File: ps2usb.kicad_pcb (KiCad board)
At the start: 2 copper layers, 62.6 x 48.2 mm, 13 parts

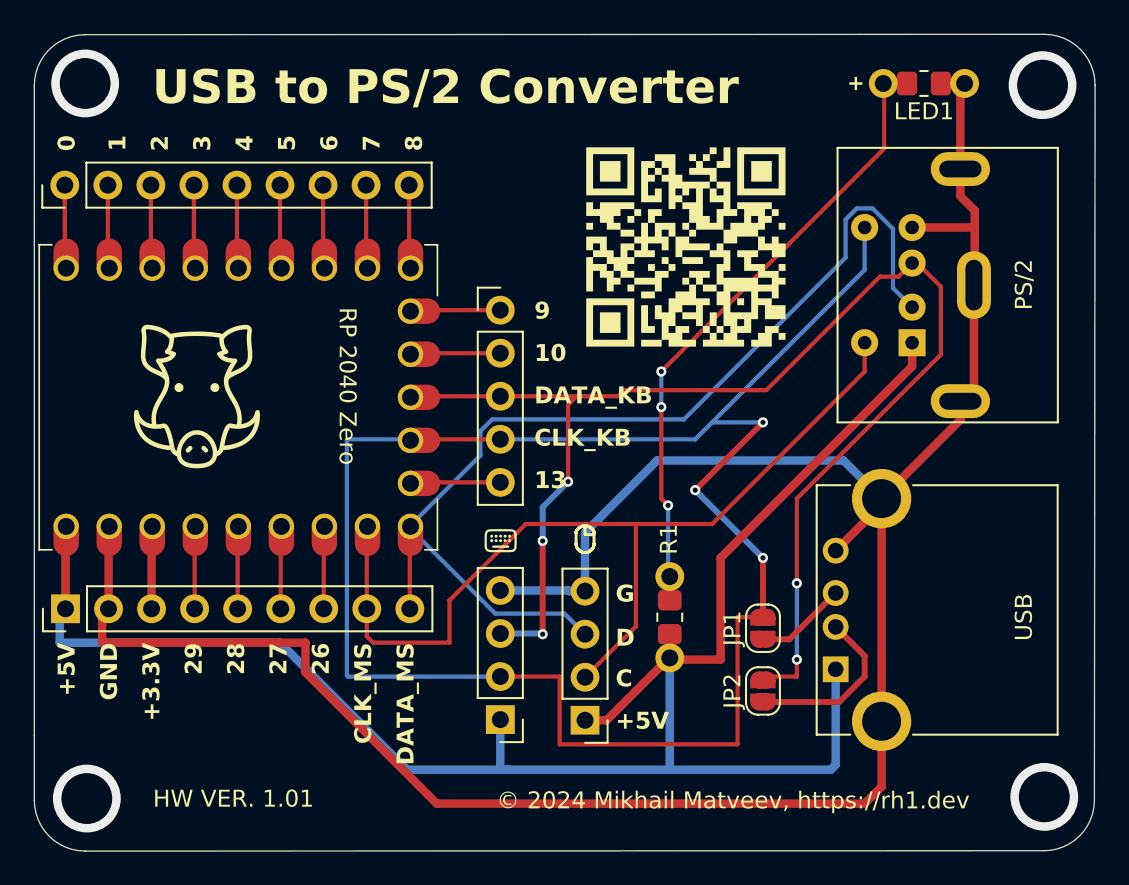
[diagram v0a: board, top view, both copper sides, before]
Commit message: HW 1.2
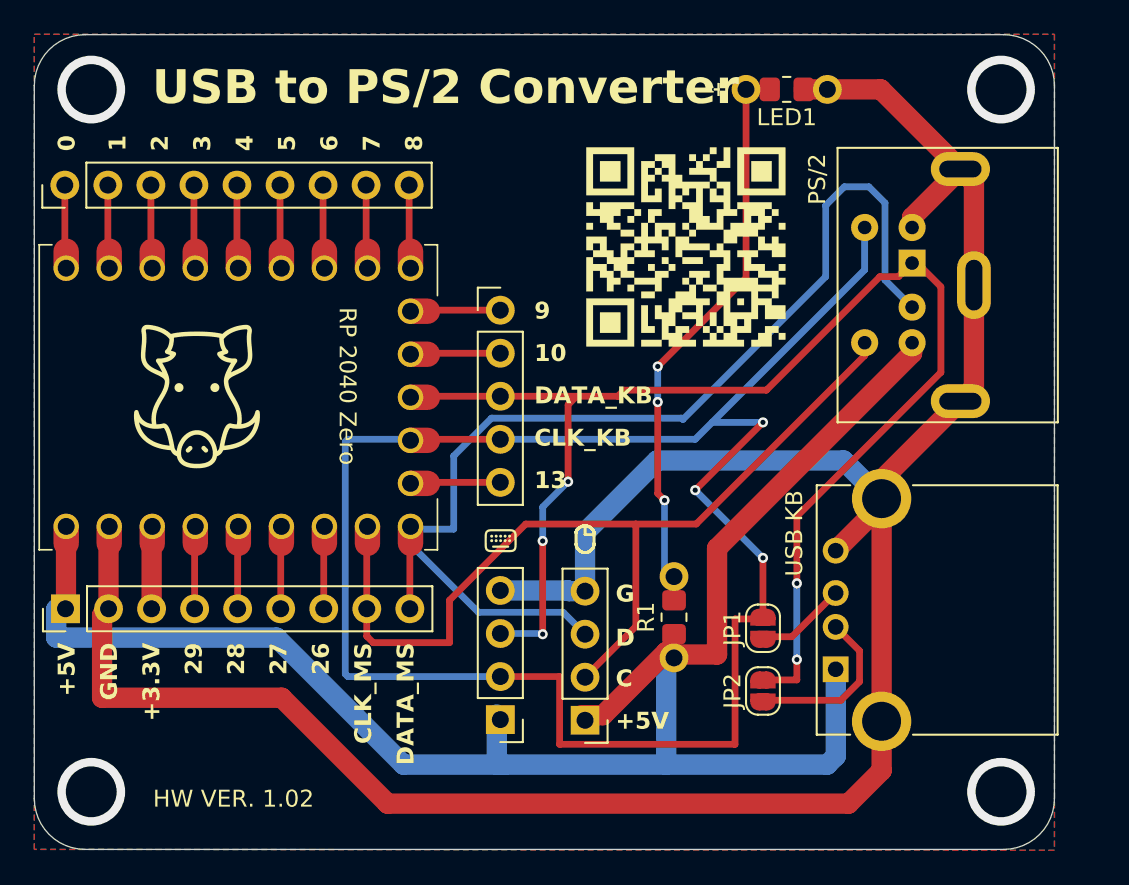
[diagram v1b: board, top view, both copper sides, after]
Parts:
- LED1, R1: footprint Resistor_SMD:R_0805_Medved -> Libs:R_0805_Medved
- PS/2: footprint Custom_Components:Connector_Mini-DIN_Female_6Pin_2rows -> Libs:Connector_Mini-DIN_Female_6Pin_2rows
- RZ1: footprint mcu:rp2040-zero-tht -> Libs:rp2040-zero-tht
- moved LED1 8.11 mm to (161.2, 79.0)
- moved R1 0.25 mm to (154.6, 110.1)
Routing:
- net GND: track 139.2 -> 146.6 mm
- net /DATA_MS: track 62.0 -> 67.1 mm
- net Net-(LED1-A): track 34.8 -> 31.1 mm
- net /CLK_MS: track 56.1 -> 55.6 mm
- added copper zone on B.Cu, net (none)
- added copper zone on F.Cu, net (none)
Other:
- board size 62.6 x 48.2 mm -> 60.2 x 48.1 mm
- board text added: "HW VER. 1.02"
- board text added: "USB KB"
- board text removed: "HW VER. 1.01"
- board text removed: "USB"
- board text removed: "© 2024 Mikhail Matveev, https://rh1.dev"
